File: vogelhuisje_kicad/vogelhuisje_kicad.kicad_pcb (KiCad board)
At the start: 2 copper layers, 17 parts, among them J1 Conn_01x02_Female, J2 Conn_01x02, J3 USB_C_Receptacle_USB2.0, J6 Conn_01x19_Female, P1 TP4056breakout, P2 GenericBoostConverter, Q1 Q_PMOS_GSD, U3 ESP32-LilyGo-T_PCIE, U4 PMS5003, U5 SD-card-reader, U6 BME280Breakout, U7 BME280Breakout

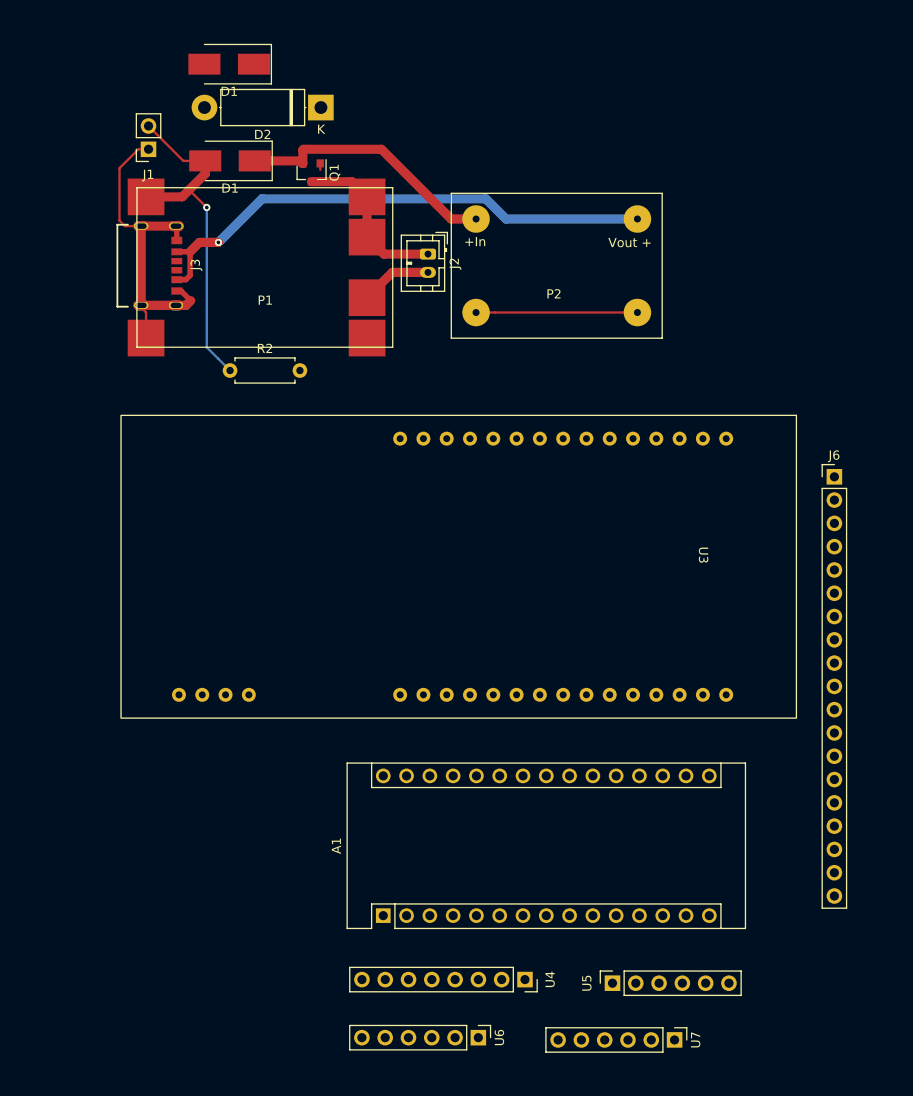
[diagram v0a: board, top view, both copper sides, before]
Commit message: PCB done with version 1
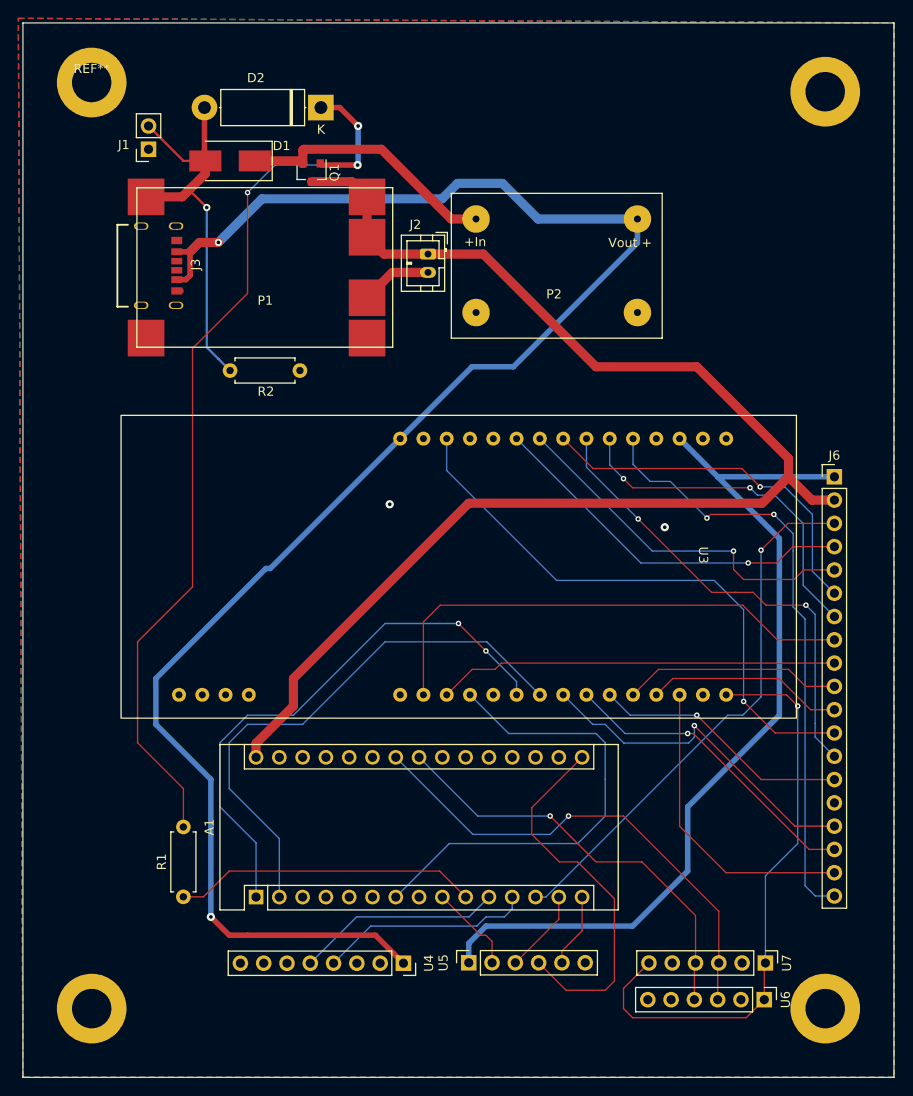
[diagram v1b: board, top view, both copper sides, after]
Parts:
- removed the D1 at (85.0, 72.0)
- added ?: , , F.Cu at (150.0, 75.0)
- added ?: , , F.Cu at (70.0, 175.0)
- added ?: , , F.Cu at (150.0, 175.0)
- added R1: -, Resistor_THT:R_Axial_DIN0207_L6.3mm_D2.5mm_P7.62mm_Horizontal, F.Cu at (80.0, 162.8)
- added REF**: MountingHole_4.3mm_M4_ISO7380_Pad, MountingHole:MountingHole_4.3mm_M4_ISO7380_Pad, F.Cu at (70.0, 74.0)
- moved U6 31.5 mm to (143.3, 174.0)
- moved U5 15.8 mm to (111.1, 170.0)
- moved A1 14.0 mm to (87.9, 162.8)
- moved U4 13.4 mm to (104.0, 170.1)
- moved U7 13.0 mm to (143.5, 170.0)
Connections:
- P1 pad 6: Net-(P1-Pad6) -> GND
- P2 pad 2: Net-(P1-Pad6) -> GND
- R2 pad 2: Net-(P1-Pad6) -> GND
- U3 pad 17: Net-(U3-Pad17) -> GND
- U6 pad 2: Net-(U3-Pad17) -> GND
- U7 pad 2: Net-(U3-Pad17) -> GND
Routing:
- net /Power Supply/Vbat: track 18.5 -> 148.5 mm
- net +5V: track 57.8 -> 185.5 mm, vias 1 -> 2
- net Net-(D2-Pad1): track 0.70 -> 102.8 mm, vias 0 -> 3
- net +3V3: track 0.00 -> 97.8 mm
- net GND: track 72.7 -> 0.73 mm, vias 0 -> 2
- net /Sensors and microcontrollers/PCLK_CAM: track 0.00 -> 66.3 mm, vias 0 -> 2
- net Net-(U3-Pad16): track 0.00 -> 64.5 mm, vias 0 -> 1
- net /Sensors and microcontrollers/XCLK_CAM: track 0.00 -> 63.5 mm, vias 0 -> 1
- net /Sensors and microcontrollers/TX_ARD: track 0.00 -> 60.3 mm, vias 0 -> 2
- net /Sensors and microcontrollers/RX_ARD: track 0.00 -> 59.9 mm
- net /Sensors and microcontrollers/LED_EN: track 0.00 -> 58.8 mm, vias 0 -> 1
- net /Sensors and microcontrollers/Y6_CAM: track 0.00 -> 55.1 mm
- net /Sensors and microcontrollers/SCL: track 0.00 -> 53.5 mm, vias 0 -> 1
- net /Sensors and microcontrollers/INT_OUT_ARD: track 0.00 -> 51.4 mm
- net /Sensors and microcontrollers/HREF_CAM: track 0.00 -> 51.1 mm, vias 0 -> 2
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- added copper zone on B.Cu, net GND
- added copper zone on F.Cu, net GND
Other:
- board outline added: 95 x 115 mm
